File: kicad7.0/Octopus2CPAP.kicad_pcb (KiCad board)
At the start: 2 copper layers, 24.3 x 21.2 mm, 9 parts, among them J1 Conn_02x05_Odd_Even, J2 Conn_01x02_Pin, Q1 AO3400A, U1 74LVC1G125

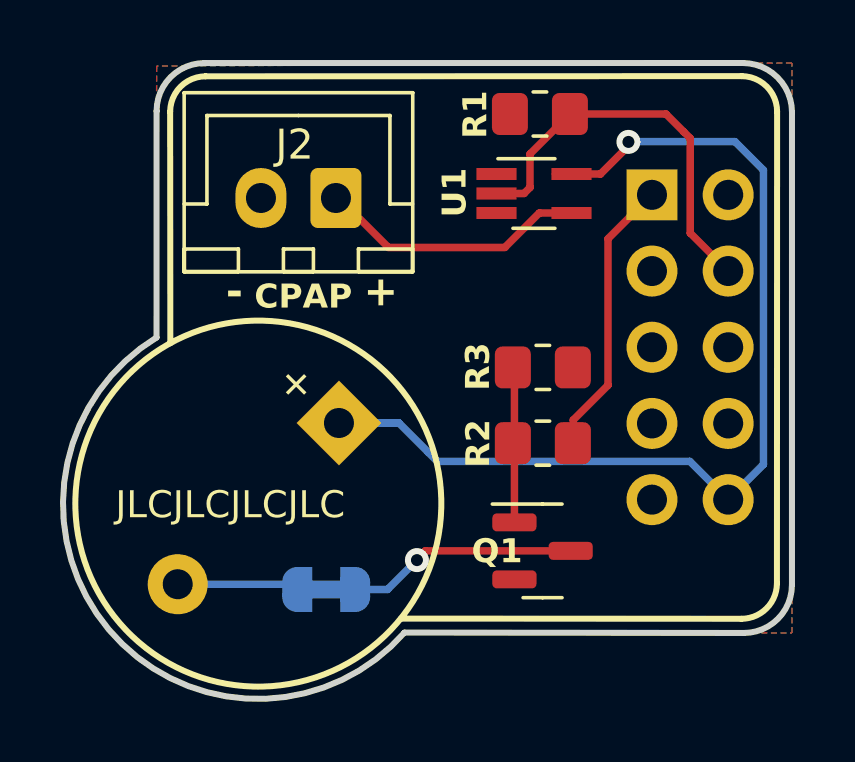
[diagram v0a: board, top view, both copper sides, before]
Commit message: finalize and release
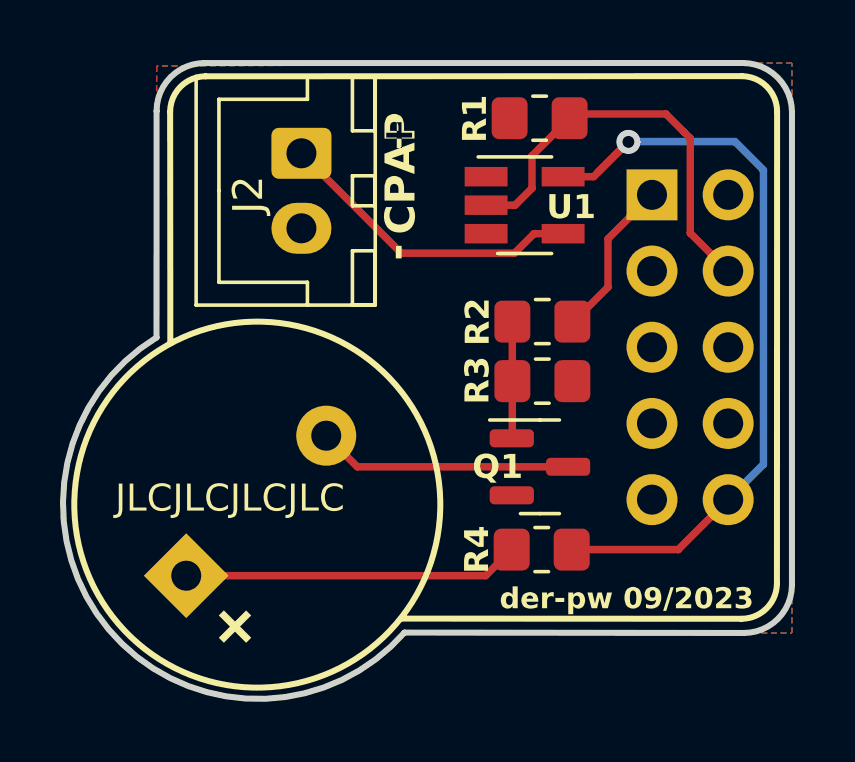
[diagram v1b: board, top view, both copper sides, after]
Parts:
- removed JP1: Jumper_2_Bridged, Jumper:SolderJumper-2_P1.3mm_Bridged_RoundedPad1.0x1.5mm
- added R4: 10R, Resistor_SMD:R_0805_2012Metric_Pad1.20x1.40mm_HandSolder, F.Cu at (195.9, 100.5)
- R2: value 330 -> 300R
- U1: footprint Package_TO_SOT_SMD:SOT-353_SC-70-5_Handsoldering -> Package_TO_SOT_SMD:SOT-23-5_HandSoldering
- moved BZ1 7.65 mm to (183.7, 101.7), turned to 45 degrees
- moved R2 4.05 mm to (195.9, 92.9)
- moved Q1 2.80 mm to (195.8, 97.8)
- moved J2 1.88 mm to (187.8, 87.3), turned to -90 degrees
- moved U1 0.50 mm to (195.3, 89.0)
- moved R3 0.46 mm to (195.9, 94.9)
- moved R1 0.14 mm to (195.8, 86.1)
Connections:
- BZ1 pad 1: +5V -> Net-(BZ1--)
- BZ1 pad 2: Net-(BZ1-+) -> /BEEPER_H
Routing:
- net Net-(BZ1--): track 0.00 -> 11.2 mm
- net +5V: track 35.7 -> 27.3 mm
- net Net-(BZ1-+): track 4.06 -> 0.00 mm
- net PE8: track 9.37 -> 5.36 mm
- net Net-(Q1-G): track 5.24 -> 3.86 mm
- net /MOT_SIG_H: track 9.44 -> 10.5 mm
- net /BEEPER_H: track 7.78 -> 8.49 mm, vias 1 -> 0
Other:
- board text added: "CPAP & Buzzer Extension for BTT Octopus"
- board text added: "der-pw 09/2023"
- board text added: "open source hardware"
- board text removed: "CPAP & Buzzer Extension for BTT Octopus (EXP1)"
- board text removed: "der-pw 08/2023"
